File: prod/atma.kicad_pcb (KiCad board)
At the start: 2 copper layers, 114.1 x 81 mm, 23 parts

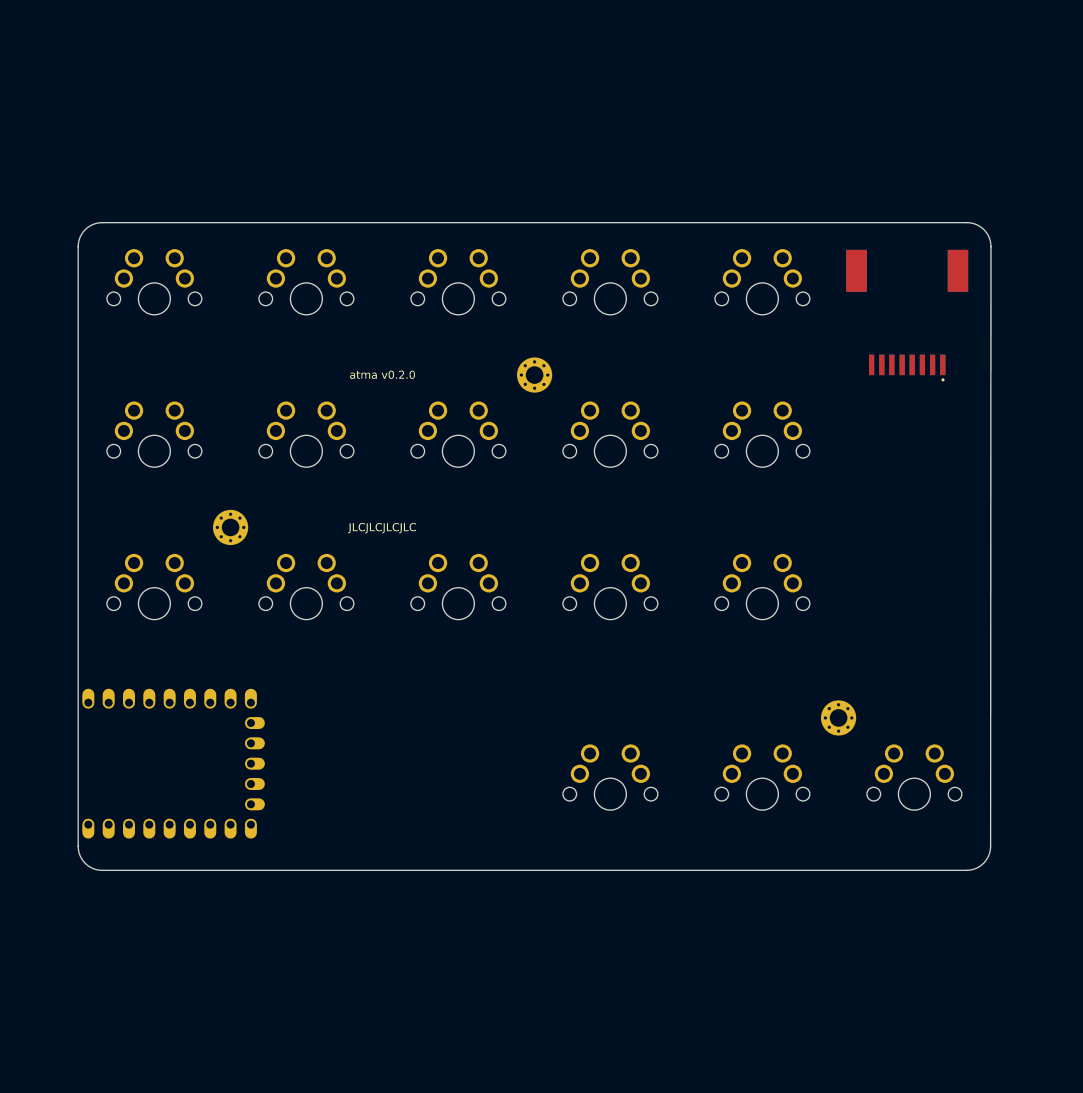
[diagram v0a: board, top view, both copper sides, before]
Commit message: finished routing
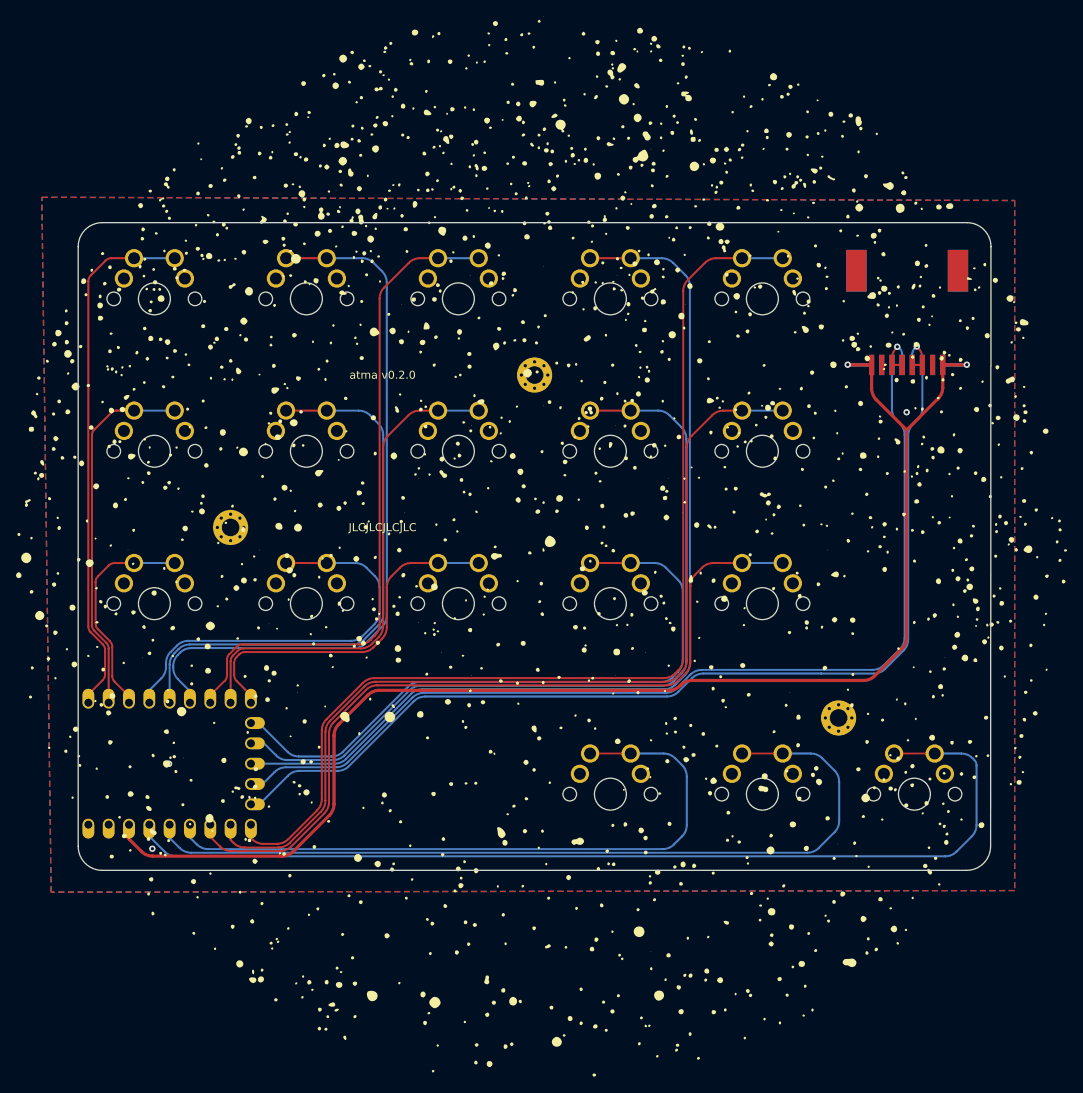
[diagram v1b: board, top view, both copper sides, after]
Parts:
- added G***: LOGO, main:north-sky-silk, F.Cu at (201.0, 145.7)
- added G***: LOGO, main:north-sky-silk, B.Cu at (198.7, 146.7)
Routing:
- net 3V3: track 0.00 -> 174.5 mm, vias 0 -> 2
- net matrix_inner_top: track 0.00 -> 131.8 mm
- net GP13: track 0.00 -> 131.1 mm, vias 0 -> 1
- net GP12: track 0.00 -> 128.9 mm, vias 0 -> 1
- net thumbfan_far_home: track 0.00 -> 124.7 mm
- net matrix_index_top: track 0.00 -> 121.5 mm
- net matrix_inner_home: track 0.00 -> 115.6 mm
- net thumbfan_home_home: track 0.00 -> 106.8 mm
- net matrix_index_home: track 0.00 -> 102.1 mm
- net matrix_inner_bottom: track 0.00 -> 98.8 mm
- net matrix_ring_top: track 0.00 -> 89.5 mm
- net thumbfan_near_home: track 0.00 -> 83.8 mm
- net matrix_middle_top: track 0.00 -> 82.1 mm
- net matrix_index_bottom: track 0.00 -> 81.7 mm
- net matrix_ring_home: track 0.00 -> 70.7 mm
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- added copper zone on B.Cu, net GND
- added copper zone on F.Cu, net GND
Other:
- net class Default removed
